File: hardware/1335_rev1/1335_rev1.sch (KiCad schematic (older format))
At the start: 20 parts, among them J1 Screw_Terminal_01x05, J2 Screw_Terminal_01x06, U1 A1335

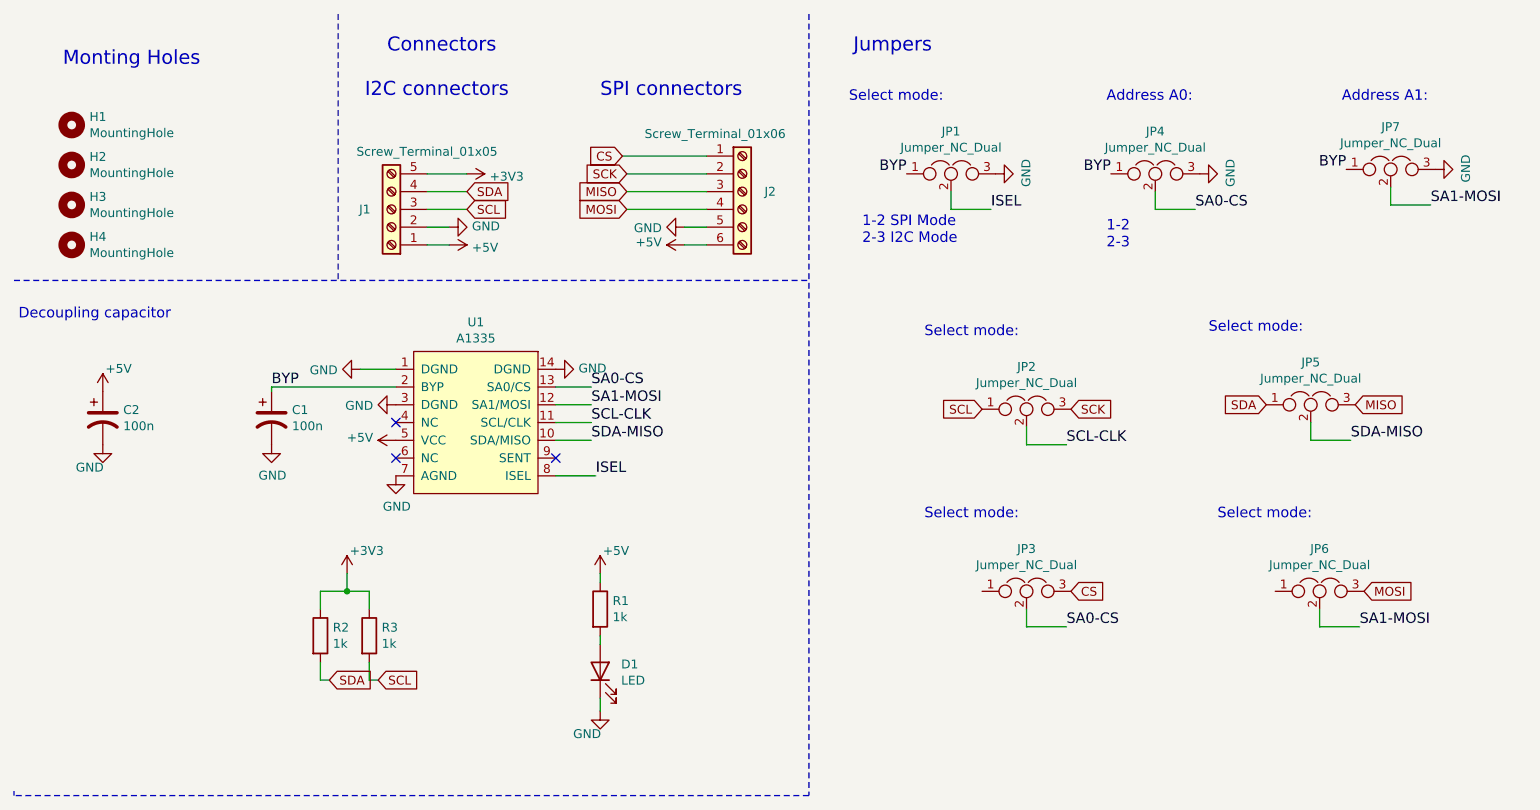
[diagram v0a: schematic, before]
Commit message: Updates
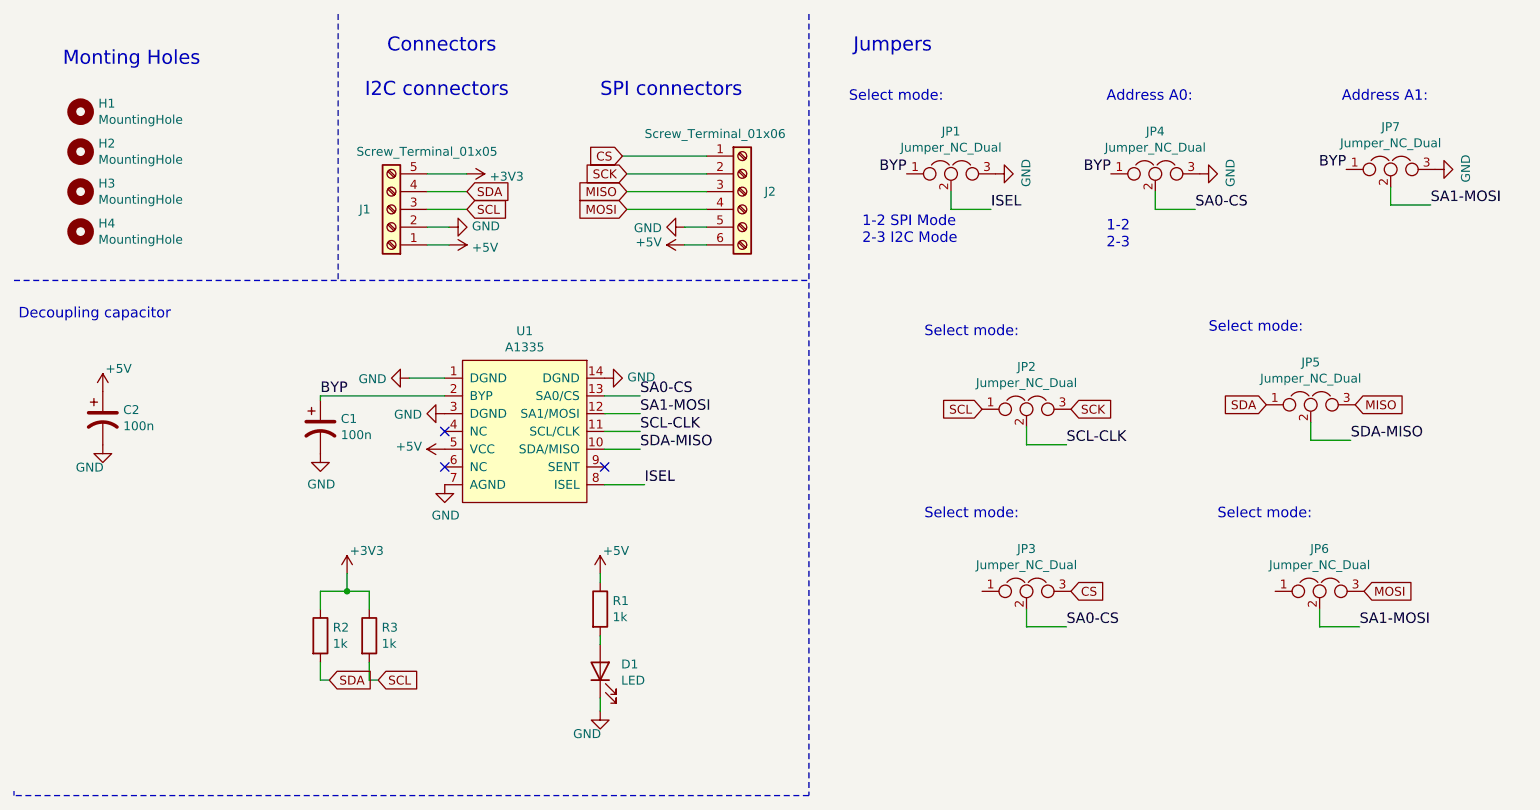
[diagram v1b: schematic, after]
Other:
- moved on the sheet: C1, H1, H2, H3, H4, U1
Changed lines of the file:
@@
 L Mechanical:MountingHole H1
 U 1 1 6046695B
-P 850 1125
-F 0 "H1" H 950 1171 50  0000 L CNN
-F 1 "MountingHole" H 950 1080 50  0000 L CNN
-F 2 "MountingHole:MountingHole_3.2mm_M3_Pad_Via" H 850 1125 50  0001 C CNN
-F 3 "~" H 850 1125 50  0001 C CNN
-	1    850  1125
+P 900 1050
+F 0 "H1" H 1000 1096 50  0000 L CNN
+F 1 "MountingHole" H 1000 1005 50  0000 L CNN
+F 2 "MountingHole:MountingHole_3.2mm_M3_Pad_Via" H 900 1050 50  0001 C CNN
+F 3 "~" H 900 1050 50  0001 C CNN
+	1    900  1050
 	1    0    0    -1
 $EndComp
@@
 L Mechanical:MountingHole H2
 U 1 1 6046714D
-P 850 1350
-F 0 "H2" H 950 1396 50  0000 L CNN
-F 1 "MountingHole" H 950 1305 50  0000 L CNN
-F 2 "MountingHole:MountingHole_3.2mm_M3_Pad_Via" H 850 1350 50  0001 C CNN
-F 3 "~" H 850 1350 50  0001 C CNN
-	1    850  1350
+P 900 1275
+F 0 "H2" H 1000 1321 50  0000 L CNN
+F 1 "MountingHole" H 1000 1230 50  0000 L CNN
+F 2 "MountingHole:MountingHole_3.2mm_M3_Pad_Via" H 900 1275 50  0001 C CNN
+F 3 "~" H 900 1275 50  0001 C CNN
+	1    900  1275
 	1    0    0    -1
 $EndComp
@@
 L Mechanical:MountingHole H3
 U 1 1 60467542
-P 850 1575
-F 0 "H3" H 950 1621 50  0000 L CNN
-F 1 "MountingHole" H 950 1530 50  0000 L CNN
-F 2 "MountingHole:MountingHole_3.2mm_M3_Pad_Via" H 850 1575 50  0001 C CNN
-F 3 "~" H 850 1575 50  0001 C CNN
-	1    850  1575
+P 900 1500
+F 0 "H3" H 1000 1546 50  0000 L CNN
+F 1 "MountingHole" H 1000 1455 50  0000 L CNN
+F 2 "MountingHole:MountingHole_3.2mm_M3_Pad_Via" H 900 1500 50  0001 C CNN
+F 3 "~" H 900 1500 50  0001 C CNN
+	1    900  1500
 	1    0    0    -1
 $EndComp
@@
 L Mechanical:MountingHole H4
 U 1 1 604678DB
-P 850 1800
-F 0 "H4" H 950 1846 50  0000 L CNN
-F 1 "MountingHole" H 950 1755 50  0000 L CNN
-F 2 "MountingHole:MountingHole_3.2mm_M3_Pad_Via" H 850 1800 50  0001 C CNN
-F 3 "~" H 850 1800 50  0001 C CNN
-	1    850  1800
+P 900 1725
+F 0 "H4" H 1000 1771 50  0000 L CNN
+F 1 "MountingHole" H 1000 1680 50  0000 L CNN
+F 2 "MountingHole:MountingHole_3.2mm_M3_Pad_Via" H 900 1725 50  0001 C CNN
+F 3 "~" H 900 1725 50  0001 C CNN
+	1    900  1725
 	1    0    0    -1
 $EndComp
@@
 L HALL:A1335 U1
 U 1 1 60468B21
-P 2475 2500
-F 0 "U1" H 3125 2765 50  0000 C CNN
-F 1 "A1335" H 3125 2674 50  0000 C CNN
-F 2 "Tssop_14:TSSOP14" H 2366 2650 50  0001 C CNN
-F 3 "" H 2366 2650 50  0001 C CNN
-	1    2475 2500
+P 2750 2550
+F 0 "U1" H 3400 2815 50  0000 C CNN
+F 1 "A1335" H 3400 2724 50  0000 C CNN
+F 2 "Tssop_14:TSSOP14" H 2641 2700 50  0001 C CNN
+F 3 "" H 2641 2700 50  0001 C CNN
+	1    2750 2550
 	1    0    0    -1
 $EndComp
@@
 Text GLabel 3950 1300 0    50   Input ~ 0
 CS
-NoConn ~ 2675 2800
-NoConn ~ 2675 3000
+NoConn ~ 2950 2850
+NoConn ~ 2950 3050
 $Comp
 L power:GND #PWR0105
 U 1 1 60476818
-P 3575 2500
-F 0 "#PWR0105" H 3575 2250 50  0001 C CNN
-F 1 "GND" V 3580 2372 50  0000 R CNN
-F 2 "" H 3575 2500 50  0001 C CNN
-F 3 "" H 3575 2500 50  0001 C CNN
-	1    3575 2500
+P 3850 2550
+F 0 "#PWR0105" H 3850 2300 50  0001 C CNN
+F 1 "GND" V 3855 2422 50  0000 R CNN
+F 2 "" H 3850 2550 50  0001 C CNN
+F 3 "" H 3850 2550 50  0001 C CNN
+	1    3850 2550
 	0    -1   -1   0
 $EndComp
@@
 L power:GND #PWR0106
 U 1 1 60477352
-P 2675 3100
-F 0 "#PWR0106" H 2675 2850 50  0001 C CNN
-F 1 "GND" H 2680 2927 50  0000 C CNN
-F 2 "" H 2675 3100 50  0001 C CNN
-F 3 "" H 2675 3100 50  0001 C CNN
-	1    2675 3100
+P 2950 3150
+F 0 "#PWR0106" H 2950 2900 50  0001 C CNN
+F 1 "GND" H 2955 2977 50  0000 C CNN
+F 2 "" H 2950 3150 50  0001 C CNN
+F 3 "" H 2950 3150 50  0001 C CNN
+	1    2950 3150
 	1    0    0    -1
 $EndComp
@@
 L power:+5V #PWR0107
 U 1 1 60479752
-P 2675 2900
-F 0 "#PWR0107" H 2675 2750 50  0001 C CNN
-F 1 "+5V" V 2690 3028 50  0000 L CNN
-F 2 "" H 2675 2900 50  0001 C CNN
-F 3 "" H 2675 2900 50  0001 C CNN
-	1    2675 2900
+P 2950 2950
+F 0 "#PWR0107" H 2950 2800 50  0001 C CNN
+F 1 "+5V" V 2965 3078 50  0000 L CNN
+F 2 "" H 2950 2950 50  0001 C CNN
+F 3 "" H 2950 2950 50  0001 C CNN
+	1    2950 2950
 	0    -1   -1   0
 $EndComp
@@
 L power:GND #PWR0108
 U 1 1 6047B24B
-P 2675 2700
-F 0 "#PWR0108" H 2675 2450 50  0001 C CNN
-F 1 "GND" V 2680 2572 50  0000 R CNN
-F 2 "" H 2675 2700 50  0001 C CNN
-F 3 "" H 2675 2700 50  0001 C CNN
-	1    2675 2700
+P 2950 2750
+F 0 "#PWR0108" H 2950 2500 50  0001 C CNN
+F 1 "GND" V 2955 2622 50  0000 R CNN
+F 2 "" H 2950 2750 50  0001 C CNN
+F 3 "" H 2950 2750 50  0001 C CNN
+	1    2950 2750
 	0    1    1    0
 $EndComp
@@
 	2350 500  2350 2000
 Wire Wire Line
-	3575 3100 3800 3100
-Text Label 3800 3100 0    59   ~ 0
+	3850 3150 4075 3150
+Text Label 4075 3150 0    59   ~ 0
 ISEL
 Text Label 6025 1600 0    59   ~ 0
 ISEL
 Wire Wire Line
-	3575 2600 3775 2600
-Wire Wire Line
-	3775 2700 3575 2700
-Wire Wire Line
-	3575 2800 3775 2800
-Wire Wire Line
-	3575 2900 3775 2900
-Text Label 1975 2600 0    59   ~ 0
+	3850 2650 4050 2650
+Wire Wire Line
+	4050 2750 3850 2750
+Wire Wire Line
+	3850 2850 4050 2850
+Wire Wire Line
+	3850 2950 4050 2950
+Text Label 2250 2650 0    59   ~ 0
 BYP
-Text Label 3775 2600 0    59   ~ 0
+Text Label 4050 2650 0    59   ~ 0
 SA0-CS
-Text Label 3775 2700 0    59   ~ 0
+Text Label 4050 2750 0    59   ~ 0
 SA1-MOSI
-Text Label 3775 2800 0    59   ~ 0
+Text Label 4050 2850 0    59   ~ 0
 SCL-CLK
-Text Label 3775 2900 0    59   ~ 0
+Text Label 4050 2950 0    59   ~ 0
 SDA-MISO
 $Comp
 L power:GND #PWR0110
 U 1 1 604837F9
-P 2475 2500
-F 0 "#PWR0110" H 2475 2250 50  0001 C CNN
-F 1 "GND" V 2480 2372 50  0000 R CNN
-F 2 "" H 2475 2500 50  0001 C CNN
-F 3 "" H 2475 2500 50  0001 C CNN
-	1    2475 2500
+P 2750 2550
+F 0 "#PWR0110" H 2750 2300 50  0001 C CNN
+F 1 "GND" V 2755 2422 50  0000 R CNN
+F 2 "" H 2750 2550 50  0001 C CNN
+F 3 "" H 2750 2550 50  0001 C CNN
+	1    2750 2550
 	0    1    1    0
 $EndComp
@@
 L power:GND #PWR0111
 U 1 1 604847D8
-P 1975 2925
-F 0 "#PWR0111" H 1975 2675 50  0001 C CNN
-F 1 "GND" H 1980 2752 50  0000 C CNN
-F 2 "" H 1975 2925 50  0001 C CNN
-F 3 "" H 1975 2925 50  0001 C CNN
-	1    1975 2925
-	1    0    0    -1
-$EndComp
-Wire Wire Line
-	1975 2600 1975 2625
-Wire Wire Line
-	1975 2600 2675 2600
-Wire Wire Line
-	2475 2500 2675 2500
+P 2250 2975
+F 0 "#PWR0111" H 2250 2725 50  0001 C CNN
+F 1 "GND" H 2255 2802 50  0000 C CNN
+F 2 "" H 2250 2975 50  0001 C CNN
+F 3 "" H 2250 2975 50  0001 C CNN
+	1    2250 2975
+	1    0    0    -1
+$EndComp
+Wire Wire Line
+	2250 2650 2250 2675
+Wire Wire Line
+	2250 2650 2950 2650
+Wire Wire Line
+	2750 2550 2950 2550
 Text Label 5550 1400 2    59   ~ 0
 BYP
@@
 L Device:CP1 C1
 U 1 1 6049E44B
-P 1975 2775
-F 0 "C1" H 2090 2821 50  0000 L CNN
-F 1 "100n" H 2090 2730 50  0000 L CNN
-F 2 "Capacitor_Tantalum_SMD:CP_EIA-1608-08_AVX-J" H 1975 2775 50  0001 C CNN
-F 3 "~" H 1975 2775 50  0001 C CNN
-	1    1975 2775
+P 2250 2825
+F 0 "C1" H 2365 2871 50  0000 L CNN
+F 1 "100n" H 2365 2780 50  0000 L CNN
+F 2 "Capacitor_Tantalum_SMD:CP_EIA-1608-08_AVX-J" H 2250 2825 50  0001 C CNN
+F 3 "~" H 2250 2825 50  0001 C CNN
+	1    2250 2825
 	1    0    0    -1
 $EndComp
@@
 	-1   0    0    1
 $EndComp
-NoConn ~ 3575 3000
+NoConn ~ 3850 3050
 Wire Notes Line
 	5000 4900 525  4900
